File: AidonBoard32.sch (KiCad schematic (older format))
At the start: 37 parts, among them J1 RJ12, M1 U-F-M5DD-Y-L, Q1 Si2301CDS-T1-GE3, Q2 MMBT3904, Q3 MMBT3904, Q4 MMBT3904, U1 AMS1117-3V3, U2 CP2102N-GQFN24, U3 ESP32-WROOM

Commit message: Fixed routing
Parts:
- J1: symbol Connector:RJ12 -> AidonBoard32-rescue:RJ12-Connector
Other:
- moved on the sheet: R6, R7, R8, R9
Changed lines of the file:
@@
 $EndComp
-Wire Wire Line
-	9450 2350 9450 2100
-Wire Wire Line
-	9450 1900 9450 1800
 Wire Wire Line
 	9450 2350 9650 2350
@@
 $EndComp
 $Comp
-L Connector:RJ12 J1
+L AidonBoard32-rescue:RJ12-Connector J1
 U 1 1 608CEFE8
 P 4250 4300
@@
 $EndComp
 $Comp
-L Device:R_Small R10
-U 1 1 60C4F049
-P 9450 2000
-F 0 "R10" H 9456 2123 50  0000 L CNN
-F 1 "10K" H 9459 1889 50  0000 L CNN
-F 2 "Resistor_SMD:R_0603_1608Metric_Pad0.98x0.95mm_HandSolder" H 9450 2000 50  0001 C CNN
-F 3 "https://datasheet.lcsc.com/lcsc/2004232132_ROHM-Semicon-ESR03EZPF1002_C510087.pdf" H 9450 2000 50  0001 C CNN
-F 4 "C510087" H 9450 2000 50  0001 C CNN "LCSC"
-	1    9450 2000
-	1    0    0    -1
-$EndComp
-$Comp
 L Device:R_Small R11
 U 1 1 60C63B88
@@
 L Device:R_Small R8
 U 1 1 5AAA8BC7
-P 9250 4450
-F 0 "R8" V 9176 4403 50  0000 L CNN
-F 1 "220" V 9325 4377 50  0000 L CNN
-F 2 "Resistor_SMD:R_0603_1608Metric_Pad0.98x0.95mm_HandSolder" H 9250 4450 50  0001 C CNN
-F 3 "" H 9250 4450 50  0001 C CNN
-F 4 "C441917" H 9250 4450 50  0001 C CNN "LCSC"
-F 5 "LED Resistors" H 9250 4450 50  0001 C CNN "Description"
-	1    9250 4450
-	0    1    1    0
-$EndComp
-Wire Wire Line
-	9500 4450 9350 4450
-Wire Wire Line
-	9050 4450 9150 4450
+P 9200 4450
+F 0 "R8" V 9126 4403 50  0000 L CNN
+F 1 "220" V 9275 4377 50  0000 L CNN
+F 2 "Resistor_SMD:R_0603_1608Metric_Pad0.98x0.95mm_HandSolder" H 9200 4450 50  0001 C CNN
+F 3 "" H 9200 4450 50  0001 C CNN
+F 4 "C441917" H 9200 4450 50  0001 C CNN "LCSC"
+F 5 "LED Resistors" H 9200 4450 50  0001 C CNN "Description"
+	1    9200 4450
+	0    1    1    0
+$EndComp
+Wire Wire Line
+	9450 4450 9300 4450
+Wire Wire Line
+	9050 4450 9100 4450
 $Comp
 L Device:LED_Small D4
@@
 L Device:R_Small R9
 U 1 1 60FFD57F
-P 9250 4700
-F 0 "R9" V 9173 4653 50  0000 L CNN
-F 1 "220" V 9328 4637 50  0000 L CNN
-F 2 "Resistor_SMD:R_0603_1608Metric_Pad0.98x0.95mm_HandSolder" H 9250 4700 50  0001 C CNN
-F 3 "" H 9250 4700 50  0001 C CNN
-F 4 "C441917" H 9250 4700 50  0001 C CNN "LCSC"
-F 5 "LED Resistors" H 9250 4700 50  0001 C CNN "Description"
-	1    9250 4700
-	0    1    1    0
-$EndComp
-Wire Wire Line
-	9050 4700 9150 4700
-Wire Wire Line
-	9500 4700 9350 4700
+P 9200 4700
+F 0 "R9" V 9123 4653 50  0000 L CNN
+F 1 "220" V 9278 4637 50  0000 L CNN
+F 2 "Resistor_SMD:R_0603_1608Metric_Pad0.98x0.95mm_HandSolder" H 9200 4700 50  0001 C CNN
+F 3 "" H 9200 4700 50  0001 C CNN
+F 4 "C441917" H 9200 4700 50  0001 C CNN "LCSC"
+F 5 "LED Resistors" H 9200 4700 50  0001 C CNN "Description"
+	1    9200 4700
+	0    1    1    0
+$EndComp
+Wire Wire Line
+	9050 4700 9100 4700
+Wire Wire Line
+	9450 4700 9300 4700
 $Comp
 L Device:LED_Small D3
@@
 $EndComp
 $Comp
+L Device:R_Small R7
+U 1 1 5AAA8B96
+P 9200 4200
+F 0 "R7" V 9125 4148 50  0000 L CNN
+F 1 "220" V 9267 4132 50  0000 L CNN
+F 2 "Resistor_SMD:R_0603_1608Metric_Pad0.98x0.95mm_HandSolder" H 9200 4200 50  0001 C CNN
+F 3 "" H 9200 4200 50  0001 C CNN
+F 4 "C441917" H 9200 4200 50  0001 C CNN "LCSC"
+F 5 "LED Resistors" H 9200 4200 50  0001 C CNN "Description"
+	1    9200 4200
+	0    1    1    0
+$EndComp
+$Comp
+L Device:R_Small R6
+U 1 1 5AAA89A6
+P 9200 3950
+F 0 "R6" V 9128 3898 50  0000 L CNN
+F 1 "220" V 9272 3885 50  0000 L CNN
+F 2 "Resistor_SMD:R_0603_1608Metric_Pad0.98x0.95mm_HandSolder" H 9200 3950 50  0001 C CNN
+F 3 "" H 9200 3950 50  0001 C CNN
+F 4 "C441917" H 9200 3950 50  0001 C CNN "LCSC"
+F 5 "LED Resistors" H 9200 3950 50  0001 C CNN "Description"
+	1    9200 3950
+	0    1    1    0
+$EndComp
+Wire Wire Line
+	10050 4700 10000 4700
+Wire Wire Line
+	9050 4200 9100 4200
+Wire Wire Line
+	9050 3950 9100 3950
+Wire Wire Line
+	9450 4200 9300 4200
+Wire Wire Line
+	9300 3950 9450 3950
+$Comp
+L power:+3.3V #PWR023
+U 1 1 5AAA9570
+P 8700 4300
+F 0 "#PWR023" H 8700 4150 50  0001 C CNN
+F 1 "+3.3V" H 8700 4440 50  0000 C CNN
+F 2 "" H 8700 4300 50  0001 C CNN
+F 3 "" H 8700 4300 50  0001 C CNN
+	1    8700 4300
+	1    0    0    -1
+$EndComp
+Text Label 9450 4200 0    60   ~ 0
+LED_RX
+Text Label 9450 3950 0    60   ~ 0
+LED_TX
+Connection ~ 8850 4200
+Wire Wire Line
+	8850 4200 8850 4450
+Wire Notes Line
+	8500 5000 11100 5000
+Wire Wire Line
+	9450 4700 9450 4450
+Connection ~ 9450 4700
+Wire Wire Line
+	9450 4700 9450 4750
+$Comp
+L power:GND #PWR0101
+U 1 1 60FFD575
+P 9450 4750
+F 0 "#PWR0101" H 9450 4500 50  0001 C CNN
+F 1 "GND" H 9450 4600 50  0000 C CNN
+F 2 "" H 9450 4750 50  0001 C CNN
+F 3 "" H 9450 4750 50  0001 C CNN
+	1    9450 4750
+	1    0    0    -1
+$EndComp
+Wire Wire Line
+	1850 4400 2050 4400
+Connection ~ 2050 4400
+Wire Wire Line
+	2050 4400 2100 4400
+$Comp
+L power:VCC #PWR0103
+U 1 1 610B3EF6
+P 10000 4700
+F 0 "#PWR0103" H 10000 4550 50  0001 C CNN
+F 1 "VCC" H 10000 4850 50  0000 C CNN
+F 2 "" H 10000 4700 50  0001 C CNN
+F 3 "" H 10000 4700 50  0001 C CNN
+	1    10000 4700
+	0    -1   -1   0
+$EndComp
+Wire Wire Line
+	2000 4350 2050 4400
+$Comp
+L power:VCC #PWR0102
+U 1 1 610A4F64
+P 2000 4350
+F 0 "#PWR0102" H 2000 4200 50  0001 C CNN
+F 1 "VCC" H 2000 4500 50  0000 C CNN
+F 2 "" H 2000 4350 50  0001 C CNN
+F 3 "" H 2000 4350 50  0001 C CNN
+	1    2000 4350
+	1    0    0    -1
+$EndComp
+$Comp
 L Device:LED_Small D2
 U 1 1 5AAA92A7
@@
 	-1   0    0    1
 $EndComp
-$Comp
-L Device:R_Small R7
-U 1 1 5AAA8B96
-P 9250 4200
-F 0 "R7" V 9175 4148 50  0000 L CNN
-F 1 "220" V 9317 4132 50  0000 L CNN
-F 2 "Resistor_SMD:R_0603_1608Metric_Pad0.98x0.95mm_HandSolder" H 9250 4200 50  0001 C CNN
-F 3 "" H 9250 4200 50  0001 C CNN
-F 4 "C441917" H 9250 4200 50  0001 C CNN "LCSC"
-F 5 "LED Resistors" H 9250 4200 50  0001 C CNN "Description"
-	1    9250 4200
-	0    1    1    0
-$EndComp
-$Comp
-L Device:R_Small R6
-U 1 1 5AAA89A6
-P 9250 3950
-F 0 "R6" V 9178 3898 50  0000 L CNN
-F 1 "220" V 9322 3885 50  0000 L CNN
-F 2 "Resistor_SMD:R_0603_1608Metric_Pad0.98x0.95mm_HandSolder" H 9250 3950 50  0001 C CNN
-F 3 "" H 9250 3950 50  0001 C CNN
-F 4 "C441917" H 9250 3950 50  0001 C CNN "LCSC"
-F 5 "LED Resistors" H 9250 3950 50  0001 C CNN "Description"
-	1    9250 3950
-	0    1    1    0
-$EndComp
-Wire Wire Line
-	10050 4700 10000 4700
-Wire Wire Line
-	9050 4200 9150 4200
-Wire Wire Line
-	9050 3950 9150 3950
-Wire Wire Line
-	9500 4200 9350 4200
-Wire Wire Line
-	9350 3950 9500 3950
-$Comp
-L power:+3.3V #PWR023
-U 1 1 5AAA9570
-P 8700 4300
-F 0 "#PWR023" H 8700 4150 50  0001 C CNN
-F 1 "+3.3V" H 8700 4440 50  0000 C CNN
-F 2 "" H 8700 4300 50  0001 C CNN
-F 3 "" H 8700 4300 50  0001 C CNN
-	1    8700 4300
-	1    0    0    -1
-$EndComp
-Text Label 9500 4200 0    60   ~ 0
-LED_RX
-Text Label 9500 3950 0    60   ~ 0
-LED_TX
-Connection ~ 8850 4200
-Wire Wire Line
-	8850 4200 8850 4450
-Wire Notes Line
-	8500 5000 11100 5000
-Wire Wire Line
-	9500 4700 9500 4450
-Connection ~ 9500 4700
-Wire Wire Line
-	9500 4700 9500 4750
-$Comp
-L power:GND #PWR0101
-U 1 1 60FFD575
-P 9500 4750
-F 0 "#PWR0101" H 9500 4500 50  0001 C CNN
-F 1 "GND" H 9500 4600 50  0000 C CNN
-F 2 "" H 9500 4750 50  0001 C CNN
-F 3 "" H 9500 4750 50  0001 C CNN
-	1    9500 4750
-	1    0    0    -1
-$EndComp
-Wire Wire Line
-	1850 4400 2050 4400
-Connection ~ 2050 4400
-Wire Wire Line
-	2050 4400 2100 4400
-$Comp
-L power:VCC #PWR0103
-U 1 1 610B3EF6
-P 10000 4700
-F 0 "#PWR0103" H 10000 4550 50  0001 C CNN
-F 1 "VCC" H 10000 4850 50  0000 C CNN
-F 2 "" H 10000 4700 50  0001 C CNN
-F 3 "" H 10000 4700 50  0001 C CNN
-	1    10000 4700
-	0    -1   -1   0
-$EndComp
-Wire Wire Line
-	2000 4350 2050 4400
-$Comp
-L power:VCC #PWR0102
-U 1 1 610A4F64
-P 2000 4350
-F 0 "#PWR0102" H 2000 4200 50  0001 C CNN
-F 1 "VCC" H 2000 4500 50  0000 C CNN
-F 2 "" H 2000 4350 50  0001 C CNN
-F 3 "" H 2000 4350 50  0001 C CNN
-	1    2000 4350
-	1    0    0    -1
-$EndComp
+Wire Wire Line
+	9450 2350 9450 2100
+Wire Wire Line
+	9450 1900 9450 1800
+$Comp
+L Device:R_Small R10
+U 1 1 60C4F049
+P 9450 2000
+F 0 "R10" H 9456 2123 50  0000 L CNN
+F 1 "10K" H 9459 1889 50  0000 L CNN
+F 2 "Resistor_SMD:R_0603_1608Metric_Pad0.98x0.95mm_HandSolder" H 9450 2000 50  0001 C CNN
+F 3 "https://datasheet.lcsc.com/lcsc/2004232132_ROHM-Semicon-ESR03EZPF1002_C510087.pdf" H 9450 2000 50  0001 C CNN
+F 4 "C510087" H 9450 2000 50  0001 C CNN "LCSC"
+	1    9450 2000
+	1    0    0    -1
+$EndComp

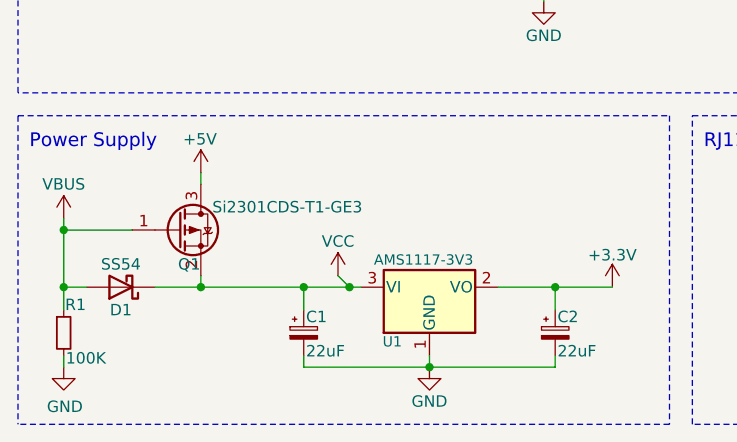
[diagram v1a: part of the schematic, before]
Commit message: Fixed small issues
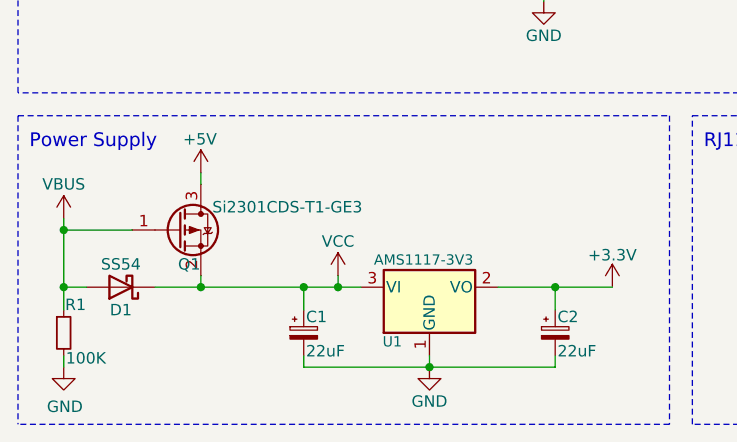
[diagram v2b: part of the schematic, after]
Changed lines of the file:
@@
 $EndComp
 Wire Wire Line
-	1850 4400 2050 4400
-Connection ~ 2050 4400
+	1850 4400 2000 4400
+Connection ~ 2000 4400
 Wire Wire Line
-	2050 4400 2100 4400
+	2000 4400 2100 4400
 $Comp
 L power:VCC #PWR0103
@@
 $EndComp
 Wire Wire Line
-	2000 4350 2050 4400
+	2000 4350 2000 4400
 $Comp
 L power:VCC #PWR0102
